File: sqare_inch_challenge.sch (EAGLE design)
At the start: 23 parts

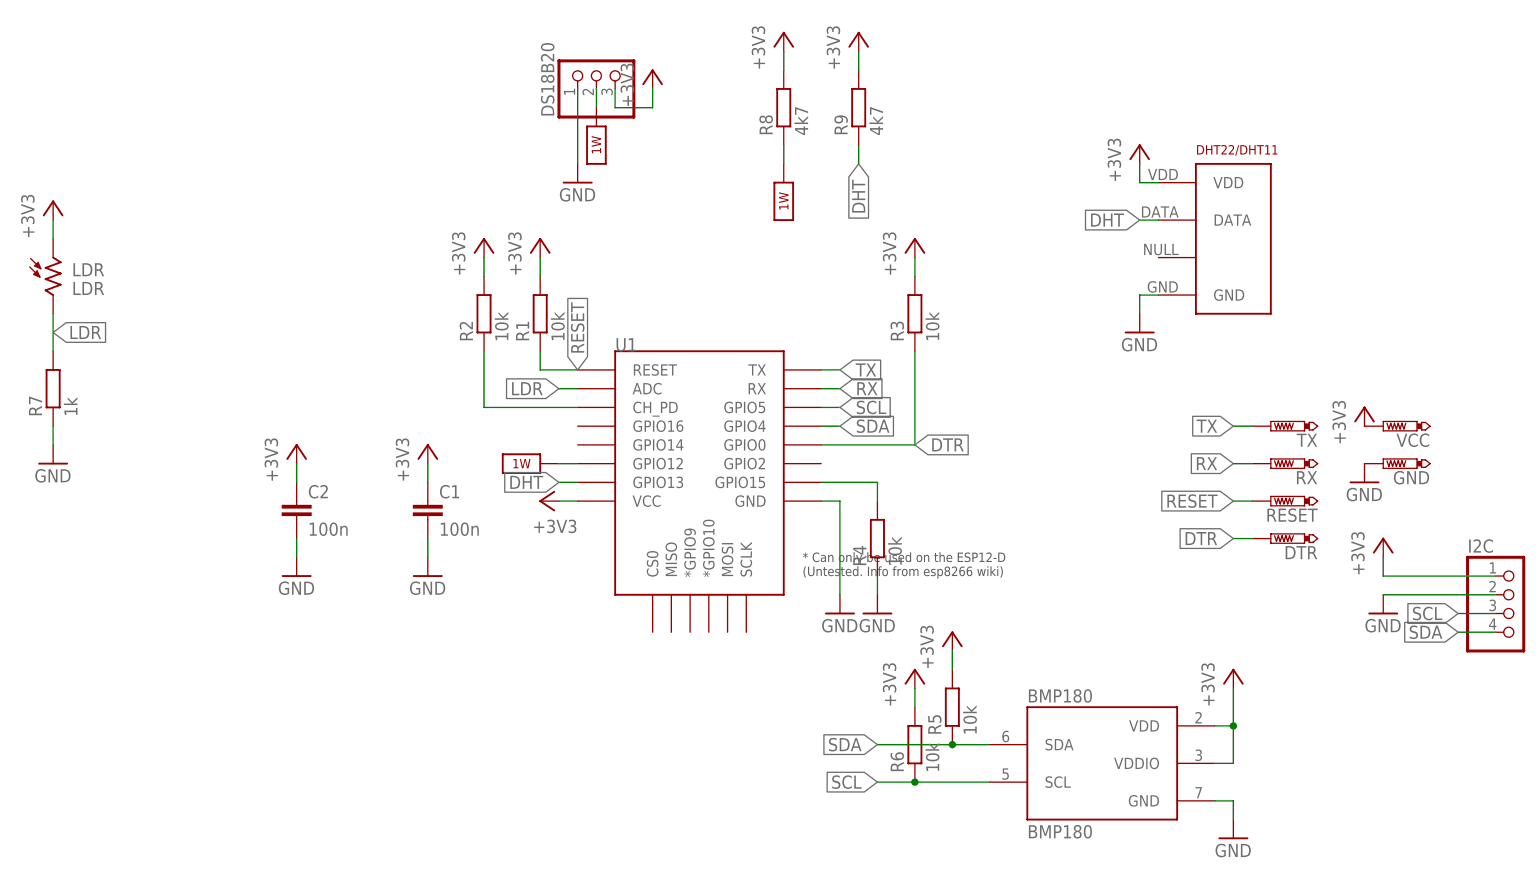
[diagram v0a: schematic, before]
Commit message: Schematic files
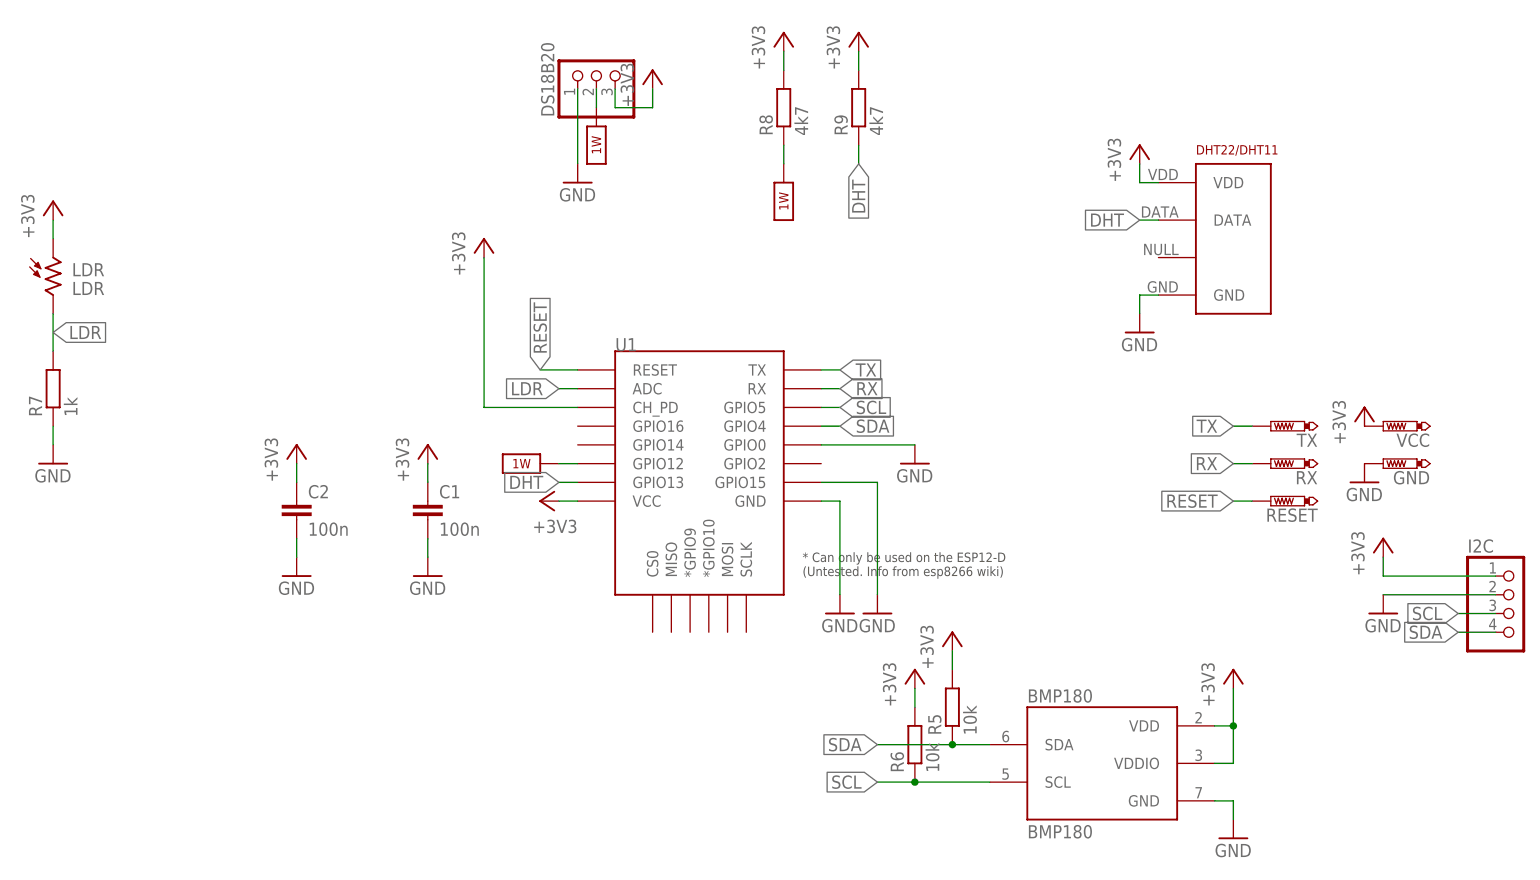
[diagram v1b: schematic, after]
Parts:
- removed DTR: PTR1TP17SQ, testpad:PTR1TP17SQ
- removed R1, R2, R3, R4: 10k, rcl:R-EU_R0805
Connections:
- removed net DTR: DTR.TP, R3.1, U1.GPIO0
- removed net N$2: R2.1, U1.CH_PD
- removed net N$4: R4.2, U1.GPIO15
- net +3V3: now also U1.CH_PD; no longer R1.2, R2.2, R3.2
- net GND: now also U1.GPIO0, U1.GPIO15; no longer R4.1
- net RESET: no longer R1.1
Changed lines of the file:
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@@
 <part name="C1" library="rcl" library_urn="urn:adsk.eagle:library:334" deviceset="C-EU" device="C0805" package3d_urn="urn:adsk.eagle:package:23617/2" value="100n"/>
 <part name="C2" library="rcl" library_urn="urn:adsk.eagle:library:334" deviceset="C-EU" device="C0805" package3d_urn="urn:adsk.eagle:package:23617/2" value="100n"/>
-<part name="R1" library="rcl" library_urn="urn:adsk.eagle:library:334" deviceset="R-EU_" device="R0805" package3d_urn="urn:adsk.eagle:package:23553/2" value="10k"/>
-<part name="R2" library="rcl" library_urn="urn:adsk.eagle:library:334" deviceset="R-EU_" device="R0805" package3d_urn="urn:adsk.eagle:package:23553/2" value="10k"/>
-<part name="R3" library="rcl" library_urn="urn:adsk.eagle:library:334" deviceset="R-EU_" device="R0805" package3d_urn="urn:adsk.eagle:package:23553/2" value="10k"/>
-<part name="R4" library="rcl" library_urn="urn:adsk.eagle:library:334" deviceset="R-EU_" device="R0805" package3d_urn="urn:adsk.eagle:package:23553/2" value="10k"/>
 <part name="+3V1" library="supply1" library_urn="urn:adsk.eagle:library:371" deviceset="+3V3" device=""/>
 <part name="+3V2" library="supply1" library_urn="urn:adsk.eagle:library:371" deviceset="+3V3" device=""/>
@@
 <part name="GND3" library="supply1" library_urn="urn:adsk.eagle:library:371" deviceset="GND" device=""/>
 <part name="+3V3" library="supply1" library_urn="urn:adsk.eagle:library:371" deviceset="+3V3" device=""/>
-<part name="+3V4" library="supply1" library_urn="urn:adsk.eagle:library:371" deviceset="+3V3" device=""/>
 <part name="+3V5" library="supply1" library_urn="urn:adsk.eagle:library:371" deviceset="+3V3" device=""/>
 <part name="DHT22/DHT11" library="Square_inch_Challange" deviceset="RHT03_DHT-22_AM2302" device=""/>
 <part name="U$1" library="1wire" deviceset="1W_SUP" device=""/>
-<part name="+3V6" library="supply1" library_urn="urn:adsk.eagle:library:371" deviceset="+3V3" device=""/>
 <part name="+3V7" library="supply1" library_urn="urn:adsk.eagle:library:371" deviceset="+3V3" device=""/>
 <part name="GND4" library="supply1" library_urn="urn:adsk.eagle:library:371" deviceset="GND" device=""/>
@@
 <part name="RX" library="testpad" library_urn="urn:adsk.eagle:library:385" deviceset="PTR1" device="TP17SQ" package3d_urn="urn:adsk.eagle:package:27977/1"/>
 <part name="RESET" library="testpad" library_urn="urn:adsk.eagle:library:385" deviceset="PTR1" device="TP17SQ" package3d_urn="urn:adsk.eagle:package:27977/1"/>
-<part name="DTR" library="testpad" library_urn="urn:adsk.eagle:library:385" deviceset="PTR1" device="TP17SQ" package3d_urn="urn:adsk.eagle:package:27977/1"/>
 <part name="BMP180" library="BMP180" deviceset="BMP180" device=""/>
 <part name="GND6" library="supply1" library_urn="urn:adsk.eagle:library:371" deviceset="GND" device=""/>
@@
 <part name="GND10" library="supply1" library_urn="urn:adsk.eagle:library:371" deviceset="GND" device=""/>
 <part name="+3V16" library="supply1" library_urn="urn:adsk.eagle:library:371" deviceset="+3V3" device=""/>
+<part name="GND11" library="supply1" library_urn="urn:adsk.eagle:library:371" deviceset="GND" device=""/>
 </parts>
 <sheets>
@@
 <instance part="C1" gate="G$1" x="5.08" y="38.1"/>
 <instance part="C2" gate="G$1" x="-12.7" y="38.1"/>
-<instance part="R1" gate="G$1" x="20.32" y="63.5" rot="R90"/>
-<instance part="R2" gate="G$1" x="12.7" y="63.5" rot="R90"/>
-<instance part="R3" gate="G$1" x="71.12" y="63.5" rot="R90"/>
-<instance part="R4" gate="G$1" x="66.04" y="33.02" rot="R90"/>
 <instance part="+3V1" gate="G$1" x="5.08" y="45.72"/>
 <instance part="+3V2" gate="G$1" x="-12.7" y="45.72"/>
@@
 <instance part="GND3" gate="1" x="-12.7" y="27.94"/>
 <instance part="+3V3" gate="G$1" x="20.32" y="38.1" rot="R90"/>
-<instance part="+3V4" gate="G$1" x="20.32" y="73.66"/>
 <instance part="+3V5" gate="G$1" x="12.7" y="73.66"/>
 <instance part="DHT22/DHT11" gate="G$1" x="114.3" y="73.66"/>
 <instance part="U$1" gate="G$1" x="22.86" y="43.18"/>
-<instance part="+3V6" gate="G$1" x="71.12" y="73.66"/>
 <instance part="+3V7" gate="G$1" x="101.6" y="86.36"/>
 <instance part="GND4" gate="1" x="101.6" y="60.96"/>
@@
 <instance part="RX" gate="G$1" x="119.38" y="43.18" rot="R90"/>
 <instance part="RESET" gate="G$1" x="119.38" y="38.1" rot="R90"/>
-<instance part="DTR" gate="G$1" x="119.38" y="33.02" rot="R90"/>
 <instance part="BMP180" gate="G$1" x="96.52" y="2.54"/>
 <instance part="GND6" gate="1" x="114.3" y="-7.62"/>
@@
 <instance part="GND10" gate="1" x="25.4" y="81.28"/>
 <instance part="+3V16" gate="G$1" x="35.56" y="96.52"/>
+<instance part="GND11" gate="1" x="71.12" y="43.18"/>
 </instances>
 <busses>
@@
 </segment>
 <segment>
-<pinref part="R4" gate="G$1" pin="1"/>
-<wire x1="66.04" y1="27.94" x2="66.04" y2="25.4" width="0.1524" layer="91"/>
 <pinref part="GND5" gate="1" pin="GND"/>
+<pinref part="U1" gate="G$1" pin="GPIO15"/>
+<wire x1="58.42" y1="40.64" x2="66.04" y2="40.64" width="0.1524" layer="91"/>
+<wire x1="66.04" y1="40.64" x2="66.04" y2="25.4" width="0.1524" layer="91"/>
 </segment>
 <segment>
@@
 <wire x1="25.4" y1="83.82" x2="25.4" y2="93.98" width="0.1524" layer="91"/>
 </segment>
+<segment>
+<pinref part="U1" gate="G$1" pin="GPIO0"/>
+<wire x1="58.42" y1="45.72" x2="71.12" y2="45.72" width="0.1524" layer="91"/>
+<pinref part="GND11" gate="1" pin="GND"/>
+</segment>
 </net>
 <net name="+3V3" class="0">
@@
 <segment>
 <pinref part="+3V5" gate="G$1" pin="+3V3"/>
-<pinref part="R2" gate="G$1" pin="2"/>
-<wire x1="12.7" y1="71.12" x2="12.7" y2="68.58" width="0.1524" layer="91"/>
-</segment>
-<segment>
-<pinref part="+3V4" gate="G$1" pin="+3V3"/>
-<pinref part="R1" gate="G$1" pin="2"/>
-<wire x1="20.32" y1="71.12" x2="20.32" y2="68.58" width="0.1524" layer="91"/>
-</segment>
-<segment>
-<pinref part="R3" gate="G$1" pin="2"/>
-<pinref part="+3V6" gate="G$1" pin="+3V3"/>
-<wire x1="71.12" y1="71.12" x2="71.12" y2="68.58" width="0.1524" layer="91"/>
+<pinref part="U1" gate="G$1" pin="CH_PD"/>
+<wire x1="12.7" y1="50.8" x2="25.4" y2="50.8" width="0.1524" layer="91"/>
+<wire x1="12.7" y1="50.8" x2="12.7" y2="71.12" width="0.1524" layer="91"/>
 </segment>
 <segment>
@@
 <pinref part="U1" gate="G$1" pin="RESET"/>
 <wire x1="25.4" y1="55.88" x2="20.32" y2="55.88" width="0.1524" layer="91"/>
-<pinref part="R1" gate="G$1" pin="1"/>
-<wire x1="20.32" y1="55.88" x2="20.32" y2="58.42" width="0.1524" layer="91"/>
-<label x="25.4" y="55.88" size="1.778" layer="95" rot="R90" xref="yes"/>
+<label x="20.32" y="55.88" size="1.778" layer="95" rot="R90" xref="yes"/>
 </segment>
 <segment>
@@
 </segment>
 </net>
-<net name="N$2" class="0">
-<segment>
-<pinref part="R2" gate="G$1" pin="1"/>
-<wire x1="12.7" y1="58.42" x2="12.7" y2="50.8" width="0.1524" layer="91"/>
-<pinref part="U1" gate="G$1" pin="CH_PD"/>
-<wire x1="12.7" y1="50.8" x2="25.4" y2="50.8" width="0.1524" layer="91"/>
-</segment>
-</net>
-<net name="N$4" class="0">
-<segment>
-<pinref part="U1" gate="G$1" pin="GPIO15"/>
-<wire x1="58.42" y1="40.64" x2="66.04" y2="40.64" width="0.1524" layer="91"/>
-<pinref part="R4" gate="G$1" pin="2"/>
-<wire x1="66.04" y1="40.64" x2="66.04" y2="38.1" width="0.1524" layer="91"/>
-</segment>
-</net>
 <net name="DHT" class="0">
 <segment>
@@
 <wire x1="116.84" y1="43.18" x2="114.3" y2="43.18" width="0.1524" layer="91"/>
 <label x="114.3" y="43.18" size="1.778" layer="95" rot="R180" xref="yes"/>
-</segment>
-</net>
-<net name="DTR" class="0">
-<segment>
-<pinref part="DTR" gate="G$1" pin="TP"/>
-<wire x1="116.84" y1="33.02" x2="114.3" y2="33.02" width="0.1524" layer="91"/>
-<label x="114.3" y="33.02" size="1.778" layer="95" rot="R180" xref="yes"/>
-</segment>
-<segment>
-<pinref part="U1" gate="G$1" pin="GPIO0"/>
-<pinref part="R3" gate="G$1" pin="1"/>
-<wire x1="58.42" y1="45.72" x2="71.12" y2="45.72" width="0.1524" layer="91"/>
-<wire x1="71.12" y1="45.72" x2="71.12" y2="58.42" width="0.1524" layer="91"/>
-<label x="71.12" y="45.72" size="1.778" layer="95" xref="yes"/>
 </segment>
 </net>
@@
 </sheet>
 </sheets>
+<errors>
+</errors>
 </schematic>
 </drawing>
